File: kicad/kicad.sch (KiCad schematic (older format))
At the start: 17 parts, among them IC1 IQRF_(DC)TR-72D, J1 Screw_Terminal_1x02, J2 Screw_Terminal_1x02, Q1 BSS138, Q2 BSS138, SW1 BondSW, U1 MeanWell_IRM-02

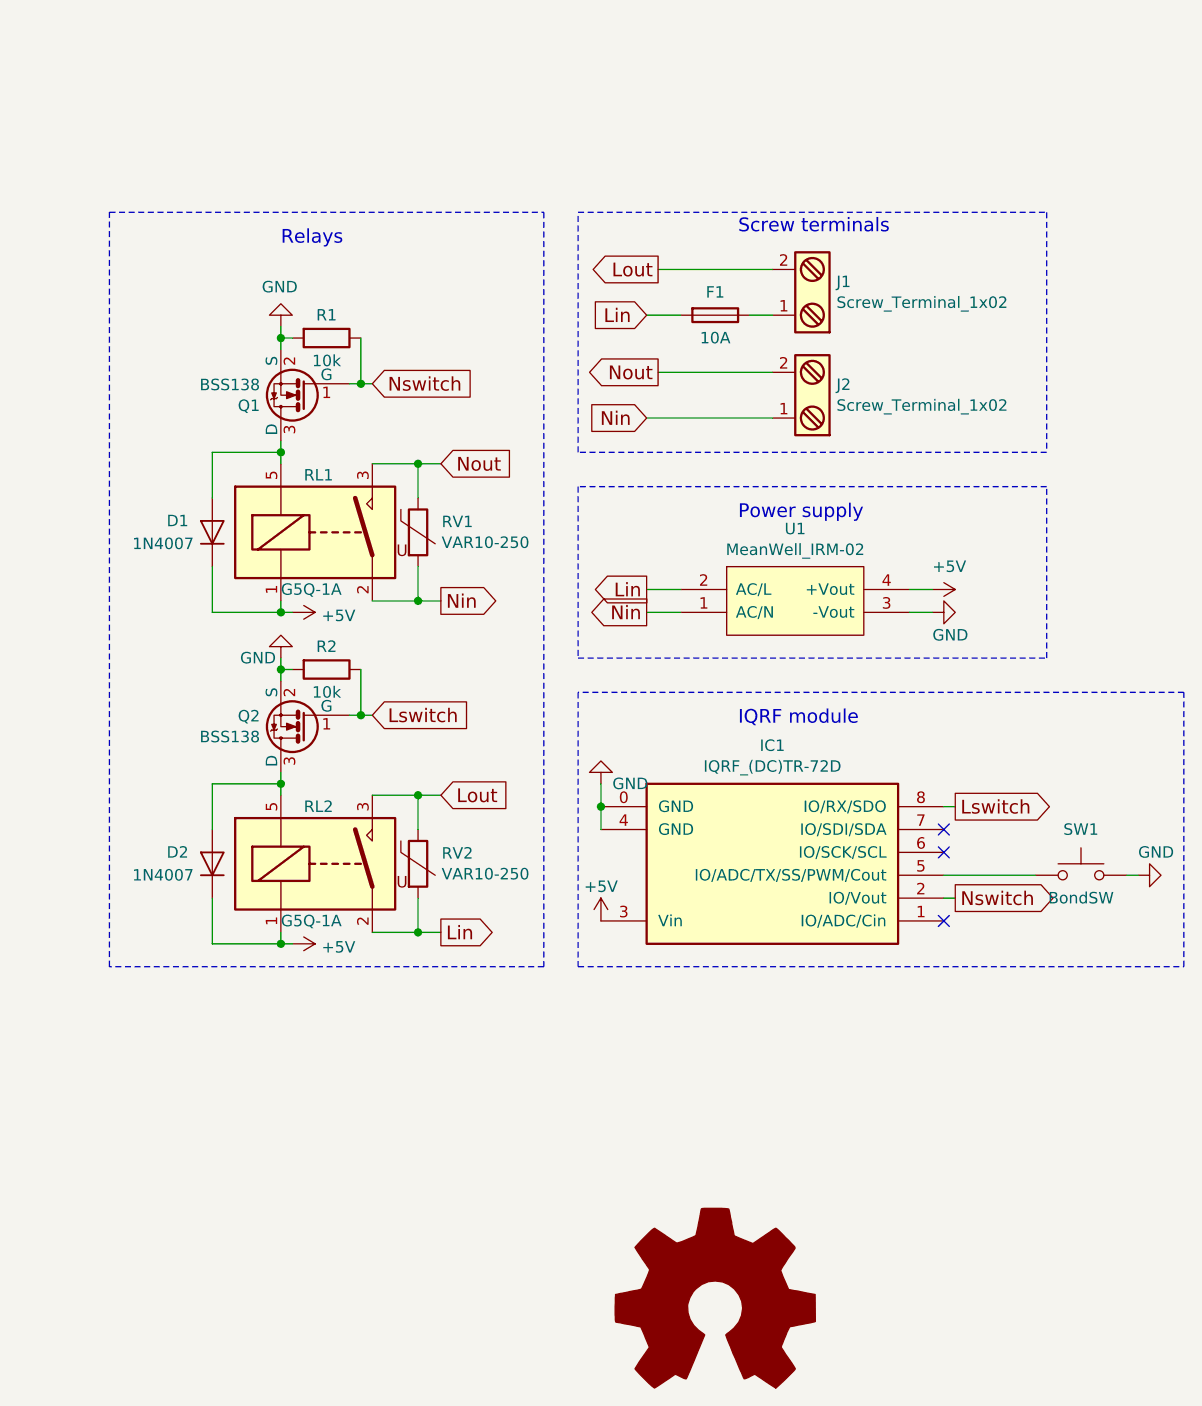
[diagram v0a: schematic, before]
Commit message: Add PCB
Signed-off-by: Roman3349 <ondracek.roman@centrum.cz>
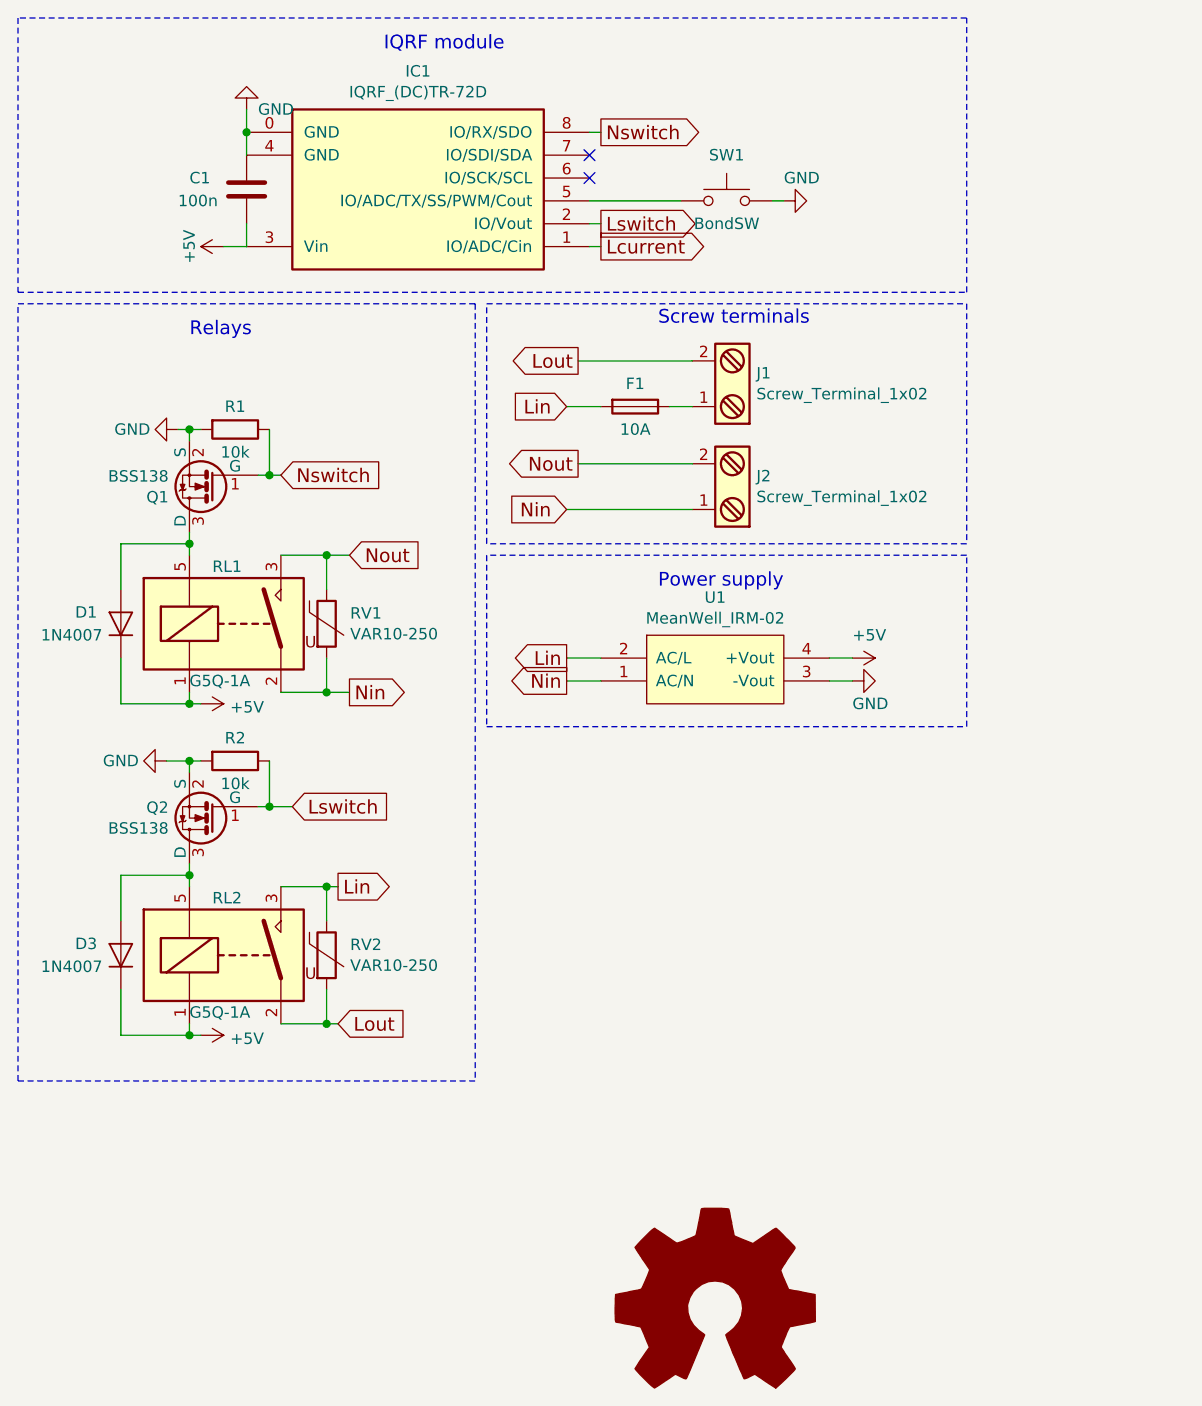
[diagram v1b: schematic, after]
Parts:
- added C1: 100n, Capacitors_SMD:C_1206_HandSoldering, symbol C
- J1, J2: footprint Terminal_Blocks:TerminalBlock_Pheonix_MKDS1.5-2pol -> Connectors_Terminal_Blocks:TerminalBlock_DG300-7.5-02P_RM7.5mm_2pol
- RV1, RV2: footprint Varistors:RV_Disc_D7_W3.5_P5 -> Varistors:RV_Disc_D12_W3.9_P7.5
- renumbered D2 to D3
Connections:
- net +5V: now also C1.2
- net GND: now also C1.1
- net Lin: now also RL2.3, RV2.1; no longer RL2.2, RV2.2
- net Lout: now also RL2.2, RV2.2; no longer RL2.3, RV2.1
- net Lswitch: now also IC1.2 (IO/Vout); no longer IC1.8 (IO/RX/SDO)
- net Nswitch: now also IC1.8 (IO/RX/SDO); no longer IC1.2 (IO/Vout)
- net Lcurrent: now reaches IC1.1 (IO/ADC/Cin)
- no-connect marks 3 -> 2
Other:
- moved on the sheet: D1, D3, F1, IC1, J1, J2, Q1, Q2, R1, R2, RL1, RL2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
